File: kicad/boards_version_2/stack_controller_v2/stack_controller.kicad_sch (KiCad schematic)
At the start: 53 parts

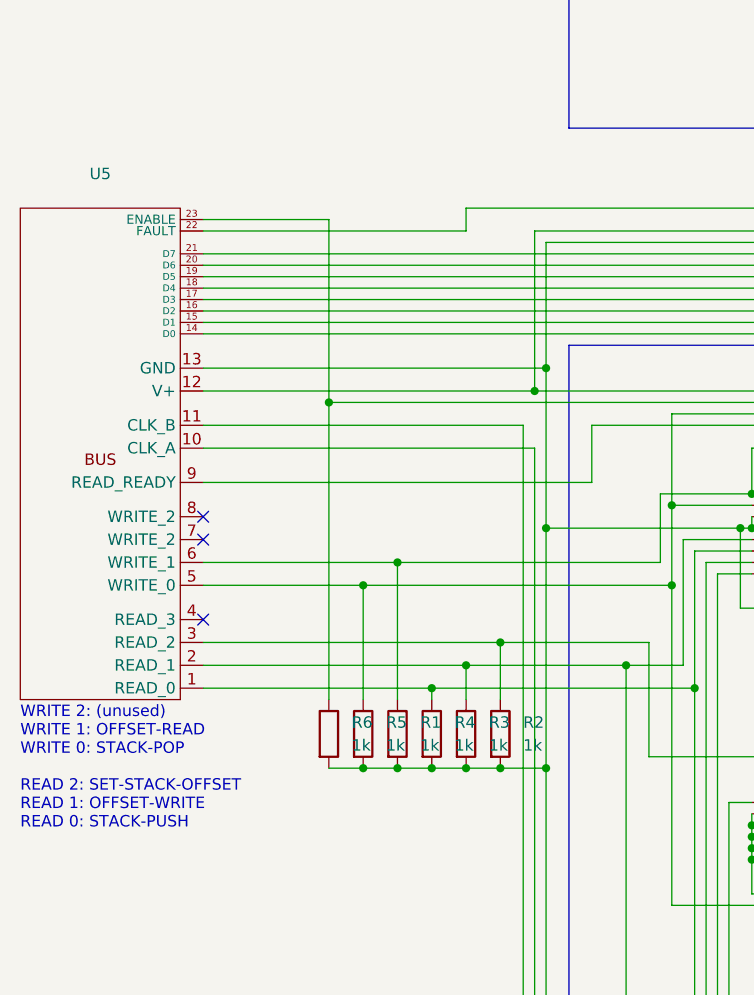
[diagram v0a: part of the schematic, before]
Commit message: Work mostly on bus
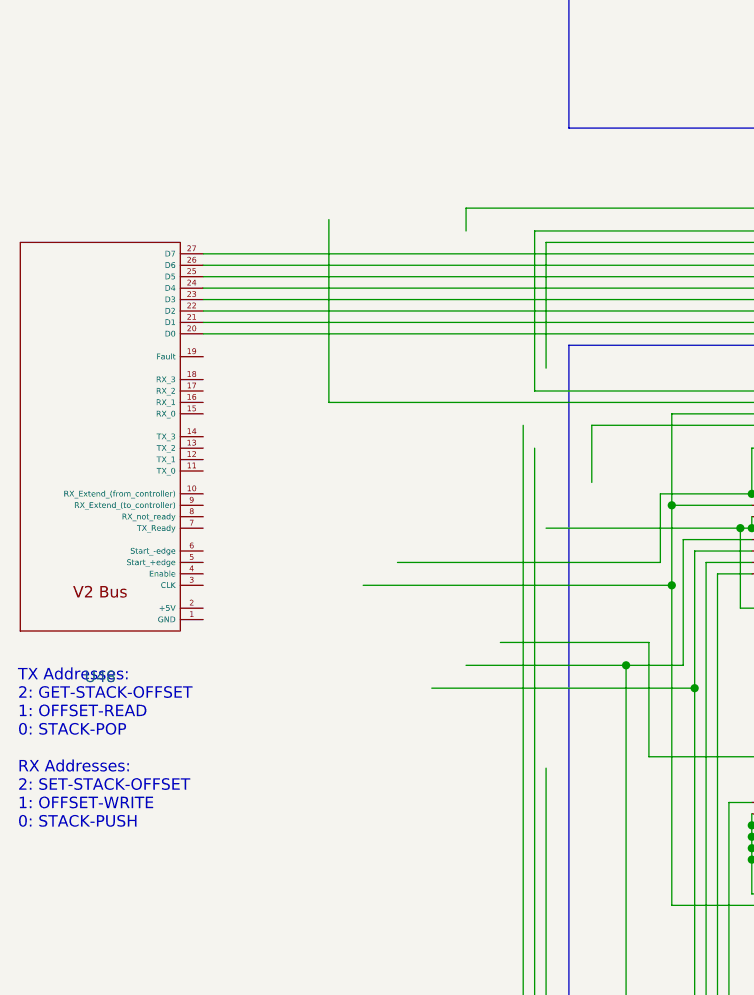
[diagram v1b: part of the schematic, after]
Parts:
- removed R1, R2, R3, R4, R5, R6: 1k, custom_footprint_library:0.4_pitch_resistor, symbol Device:R
- removed U5: ~, Connector_PinHeader_2.54mm:PinHeader_1x23_P2.54mm_Vertical, symbol custom_symbol_lib:bus_edge_connector
- added U48: ~, Connector_PinHeader_2.54mm:PinHeader_1x27_P2.54mm_Vertical, symbol custom_symbol_lib:bus_v2
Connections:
- net at U1.7 (C_IN), U1.8 (GND), U10.14 (GND)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: no longer U24.7 (GND), U25.5 (1A), U25.6 (1B), U25.7 (GND), U26.1 (OE#), U26.10 (GND), U26.9 (D7), U27.7 (GND), U28.7 (GND), U31.11 (I4), U31.13 (I5), U31.3 (I1), U31.5 (I2), U31.7 (GND), U31.9 (I3), U47.10 (4A), U47.12 (3B), U47.13 (3A), U47.4 (2A), U47.5 (2B), U47.7 (GND), U47.9 (4B), U9.1 (OE#), U9.10 (GND)
- net at U18.2 (D0), U29.19 (Q0), U30.2 (D0): now also U48.20 (D0)
- net at U18.3 (D1), U29.18 (Q1), U30.3 (D1): now also U48.21 (D1)
- net at U18.4 (D2), U29.17 (Q2), U30.4 (D2): now also U48.22 (D2)
- net at U18.5 (D3), U29.16 (Q3), U30.5 (D3): now also U48.23 (D3)
- net at U18.6 (D4), U29.15 (Q4), U30.6 (D4): now also U48.24 (D4)
- net at U18.7 (D5), U29.14 (Q5), U30.7 (D5): now also U48.25 (D5)
- net at U18.8 (D6), U29.13 (Q6), U30.8 (D6): now also U48.26 (D6)
- net at U18.9 (D7), U29.12 (Q7), U30.9 (D7): now also U48.27 (D7)
- new net: U25.5 (1A), U25.6 (1B), U25.7 (GND)
- new net: U24.7 (GND), U26.1 (OE#), U26.10 (GND), U26.9 (D7), U27.7 (GND), U28.7 (GND), U31.11 (I4), U31.13 (I5), U31.3 (I1), U31.5 (I2), U31.7 (GND), U31.9 (I3), U47.10 (4A), U47.12 (3B), U47.13 (3A), U47.4 (2A), U47.5 (2B), U47.7 (GND), U47.9 (4B), U9.1 (OE#), U9.10 (GND)
- no-connect marks 16 -> 13
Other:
- note added: "TX Addresses: 2: GET-STACK-OFFSET 1: OFFSET-READ 0: STACK-POP RX Addresses: 2: SET-STACK-OFFSET 1: OFFSET-WRITE 0: STACK-PUSH"
- note removed: "WRITE 2: (unused) WRITE 1: OFFSET-READ WRITE 0: STACK-POP READ 2: SET-STACK-OFFSET READ 1: OFFSET-WRITE READ 0: STACK-PUSH"
